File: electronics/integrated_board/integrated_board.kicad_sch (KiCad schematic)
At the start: 67 parts, among them CON1 BARREL_JACK, J1 to_rotary_encoder3(12,13), J13 to_motor1(15,2,0,4), J15 to_motor2 (16,17,5,18), J17 to_motor3 (19,21,22,23), J2 to_rotary_encoder3, J5 to_rotary_encoder2 (14,27), P1 Conn_01x02, P10 Conn_01x02, P15 Conn_01x02, P16 UART, P2 LCD, P4 io, Q1 2N7000, Q2 2N7000, Q3 2N7000, Q4 2N7000, Q5 2N7000, Q6 2N7000, SW1 SW_Push, SW2 SW_Push, U1 ULN2003, U2 ULN2003, U3 LM2596T-5, U4 ESP32-DEVKITC-32D

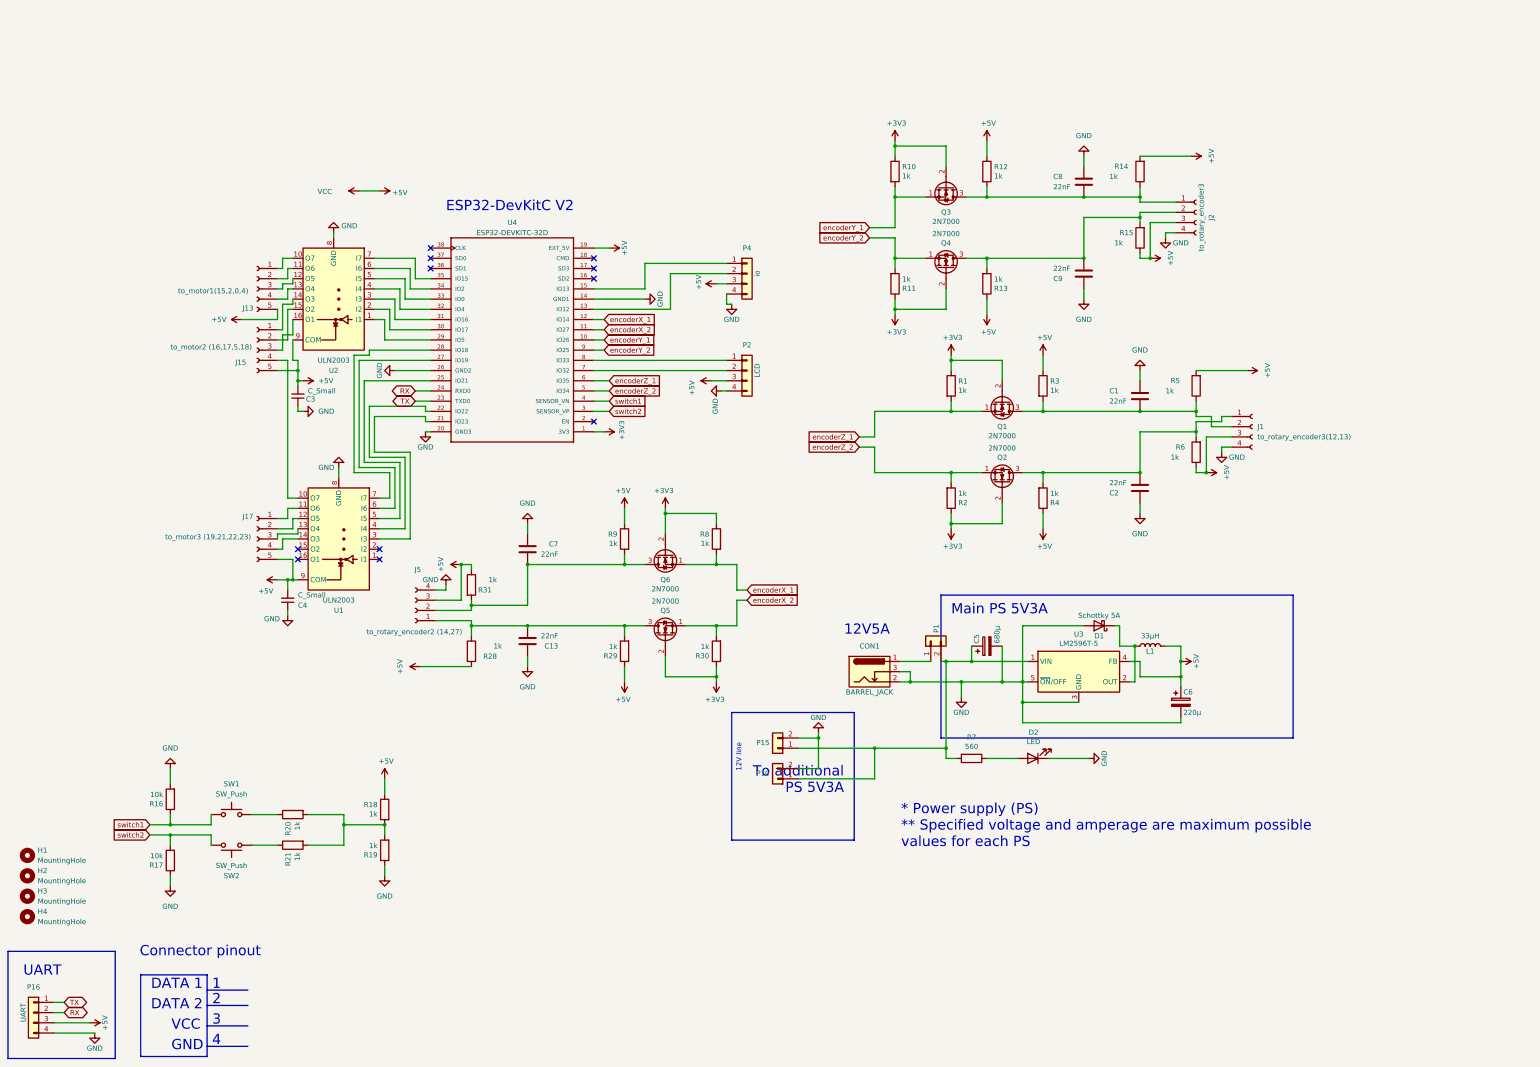
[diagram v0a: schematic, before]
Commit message: finish revision of integrated pcb board, create production files
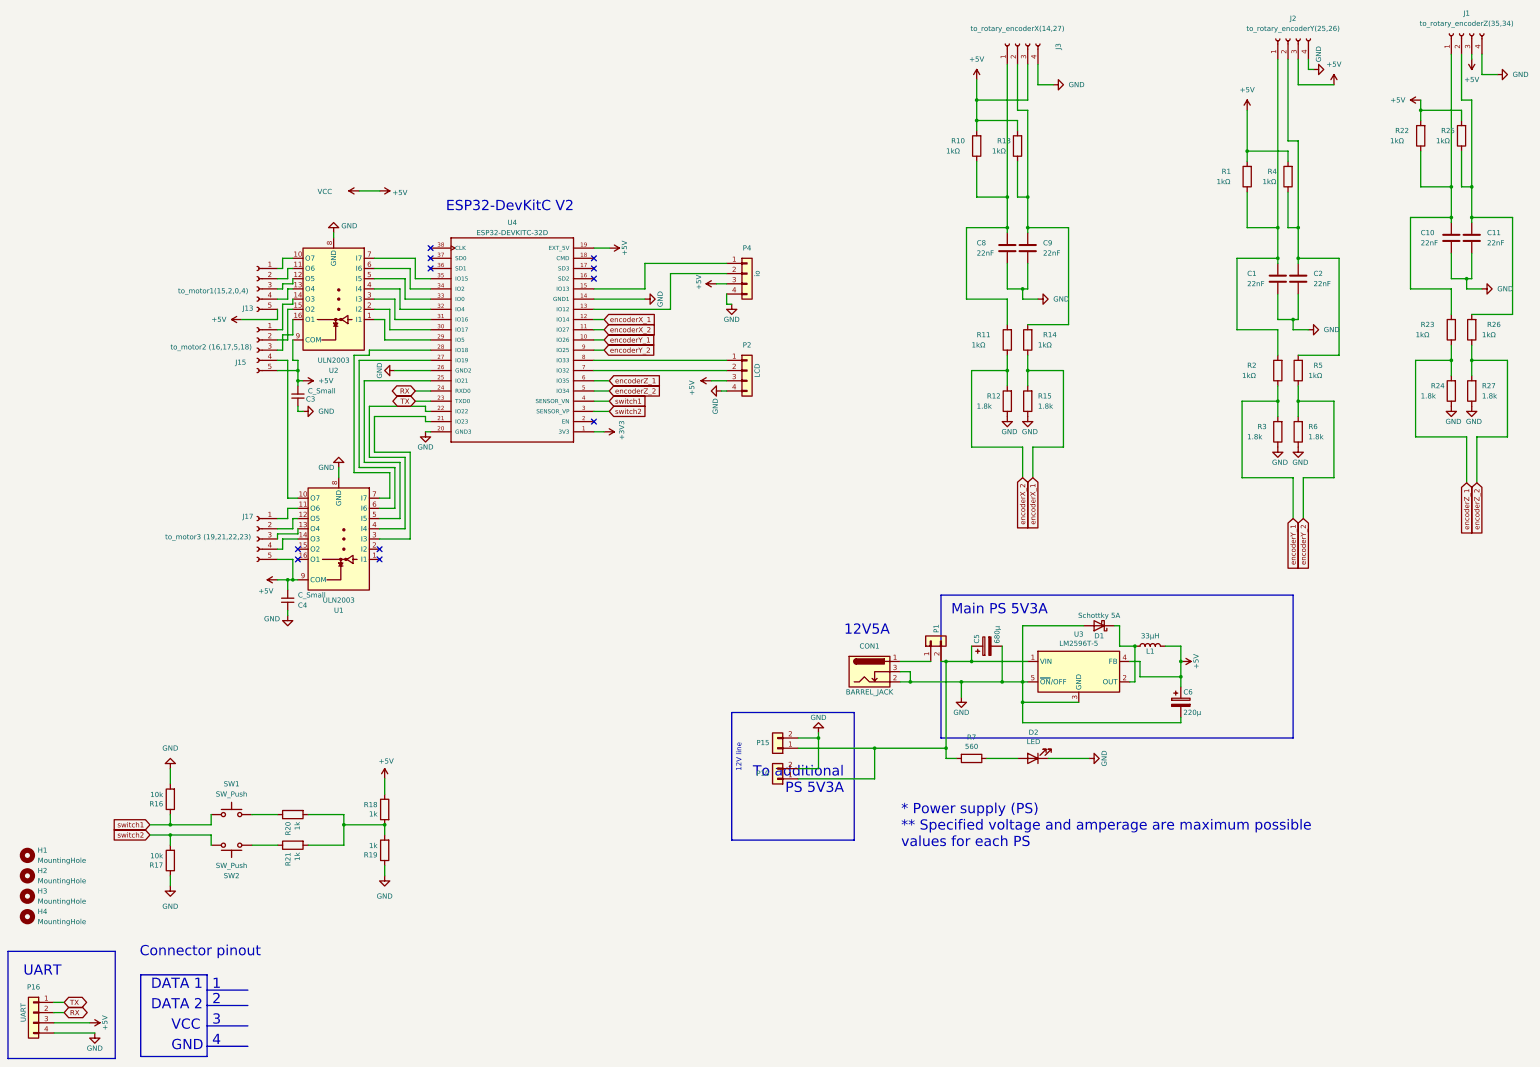
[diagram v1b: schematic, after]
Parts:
- removed C13, C7: 22nF, Capacitor_THT:CP_Radial_D4.0mm_P2.00mm, symbol Device:C
- removed J5: to_rotary_encoder2 (14,27), Connector_JST:JST_XH_B4B-XH-A_1x04_P2.50mm_Vertical, symbol Connector:Conn_01x04_Female
- removed Q1, Q2, Q3, Q4, Q5, Q6: 2N7000, Package_TO_SOT_THT:TO-92_Inline_Wide, symbol Transistor_FET:2N7000
- removed R28, R31: 1k, Resistor_THT:R_Axial_DIN0309_L9.0mm_D3.2mm_P12.70mm_Horizontal, symbol Device:R
- removed R29, R30, R8, R9: 1k, Resistor_THT:R_Axial_DIN0411_L9.9mm_D3.6mm_P12.70mm_Horizontal, symbol Device:R
- added C10, C11: 22nF, Capacitor_THT:C_Disc_D6.0mm_W4.4mm_P5.00mm, symbol Device:C
- added J3: to_rotary_encoderX(14,27), Connector_JST:JST_XH_B4B-XH-A_1x04_P2.50mm_Vertical, symbol Connector:Conn_01x04_Female
- added R22, R23, R25, R26: 1kΩ, Resistor_THT:R_Axial_DIN0309_L9.0mm_D3.2mm_P12.70mm_Horizontal, symbol Device:R
- added R24, R27: 1.8k, Resistor_THT:R_Axial_DIN0309_L9.0mm_D3.2mm_P12.70mm_Horizontal, symbol Device:R
- C1, C2, C8, C9: footprint Capacitor_THT:CP_Radial_D4.0mm_P2.00mm -> Capacitor_THT:C_Disc_D6.0mm_W4.4mm_P5.00mm
- J1: value to_rotary_encoder3(12,13) -> to_rotary_encoderZ(35,34)
- J2: value to_rotary_encoder3 -> to_rotary_encoderY(25,26)
- R1, R10, R11, R13, R2, R4: value 1k -> 1kΩ; footprint Resistor_THT:R_Axial_DIN0411_L9.9mm_D3.6mm_P12.70mm_Horizontal -> Resistor_THT:R_Axial_DIN0309_L9.0mm_D3.2mm_P12.70mm_Horizontal
- R12, R3: value 1k -> 1.8k; footprint Resistor_THT:R_Axial_DIN0411_L9.9mm_D3.6mm_P12.70mm_Horizontal -> Resistor_THT:R_Axial_DIN0309_L9.0mm_D3.2mm_P12.70mm_Horizontal
- R14, R5: value 1k -> 1kΩ
- R15, R6: value 1k -> 1.8k
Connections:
- net +3V3: no longer R1.1, R10.1, R11.1, R2.1
- net +5V: now also R1.2, R10.2, R13.2, R4.2, J3.3 (Pin_3), R22.2, R25.2; no longer R12.1, R13.1, R14.2, R15.1, R3.1, R4.1, R5.2, R6.1
- net GND: now also C1.1, C2.1, C8.1, C9.1, R12.1, R15.1, R3.1, R6.1, C10.1, C11.1, J3.4 (Pin_4), R24.1, R27.1; no longer C1.2, C2.2, C8.2, C9.2
- net encoderX_1: now also R14.1, R15.2
- net encoderX_2: now also R11.1, R12.2
- net encoderY_1: now also R2.1, R3.2; no longer R10.2
- net encoderY_2: now also R5.1, R6.2; no longer R11.2
- net encoderZ_1: now also R23.1, R24.2; no longer R1.2
- net encoderZ_2: now also R26.1, R27.2; no longer R2.2
- new net: C10.2, J1.1 (Pin_1), R22.1, R23.2
- new net: C11.2, J1.2 (Pin_2), R25.1, R26.2
- new net: C8.2, J3.1 (Pin_1), R10.1, R11.2
- new net: C2.2, J2.2 (Pin_2), R4.1, R5.2
- new net: C9.2, J3.2 (Pin_2), R13.1, R14.2
- new net: C1.2, J2.1 (Pin_1), R1.1, R2.2
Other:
- moved on the sheet: J1, J2
